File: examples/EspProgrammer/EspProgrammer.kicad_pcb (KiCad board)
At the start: 2 copper layers, 35 x 12 mm, 27 parts

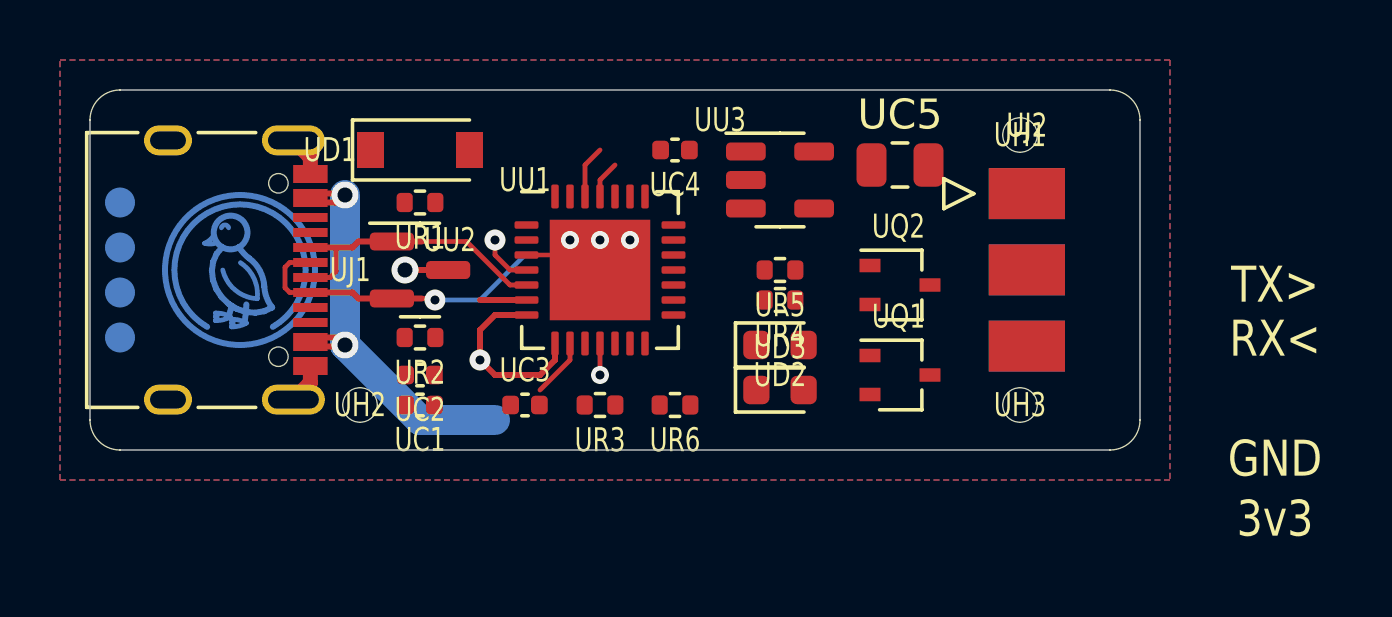
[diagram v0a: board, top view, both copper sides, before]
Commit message: d e n s i t y
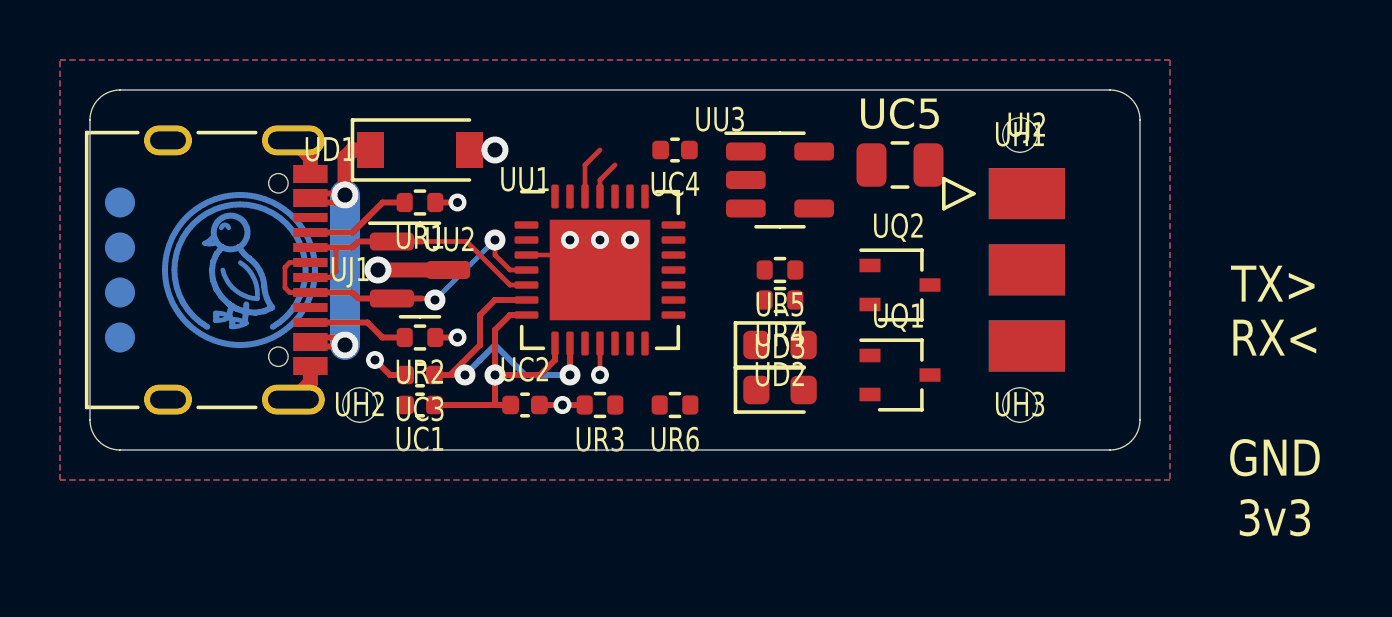
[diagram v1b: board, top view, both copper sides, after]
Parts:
- moved UC2 3.64 mm to (148.5, 52.5), turned to 0 degrees
- moved UC3 3.64 mm to (145.0, 51.5), turned to 180 degrees
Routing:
- net usbconv.ic.vdd: track 3.51 -> 10.6 mm, vias 0 -> 2
- net gnd: track 7.94 -> 12.5 mm, vias 4 -> 9
- net usb_uart.conn.A5: track 0.00 -> 3.56 mm
- net usb_uart.conn.B5: track 0.00 -> 3.35 mm
- net usb_chain_0.d_P: track 13.5 -> 12.7 mm
